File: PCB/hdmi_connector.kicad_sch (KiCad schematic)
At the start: 4 parts, among them J4 HDMI_A_1.4, U11 PTN3360DBS_518

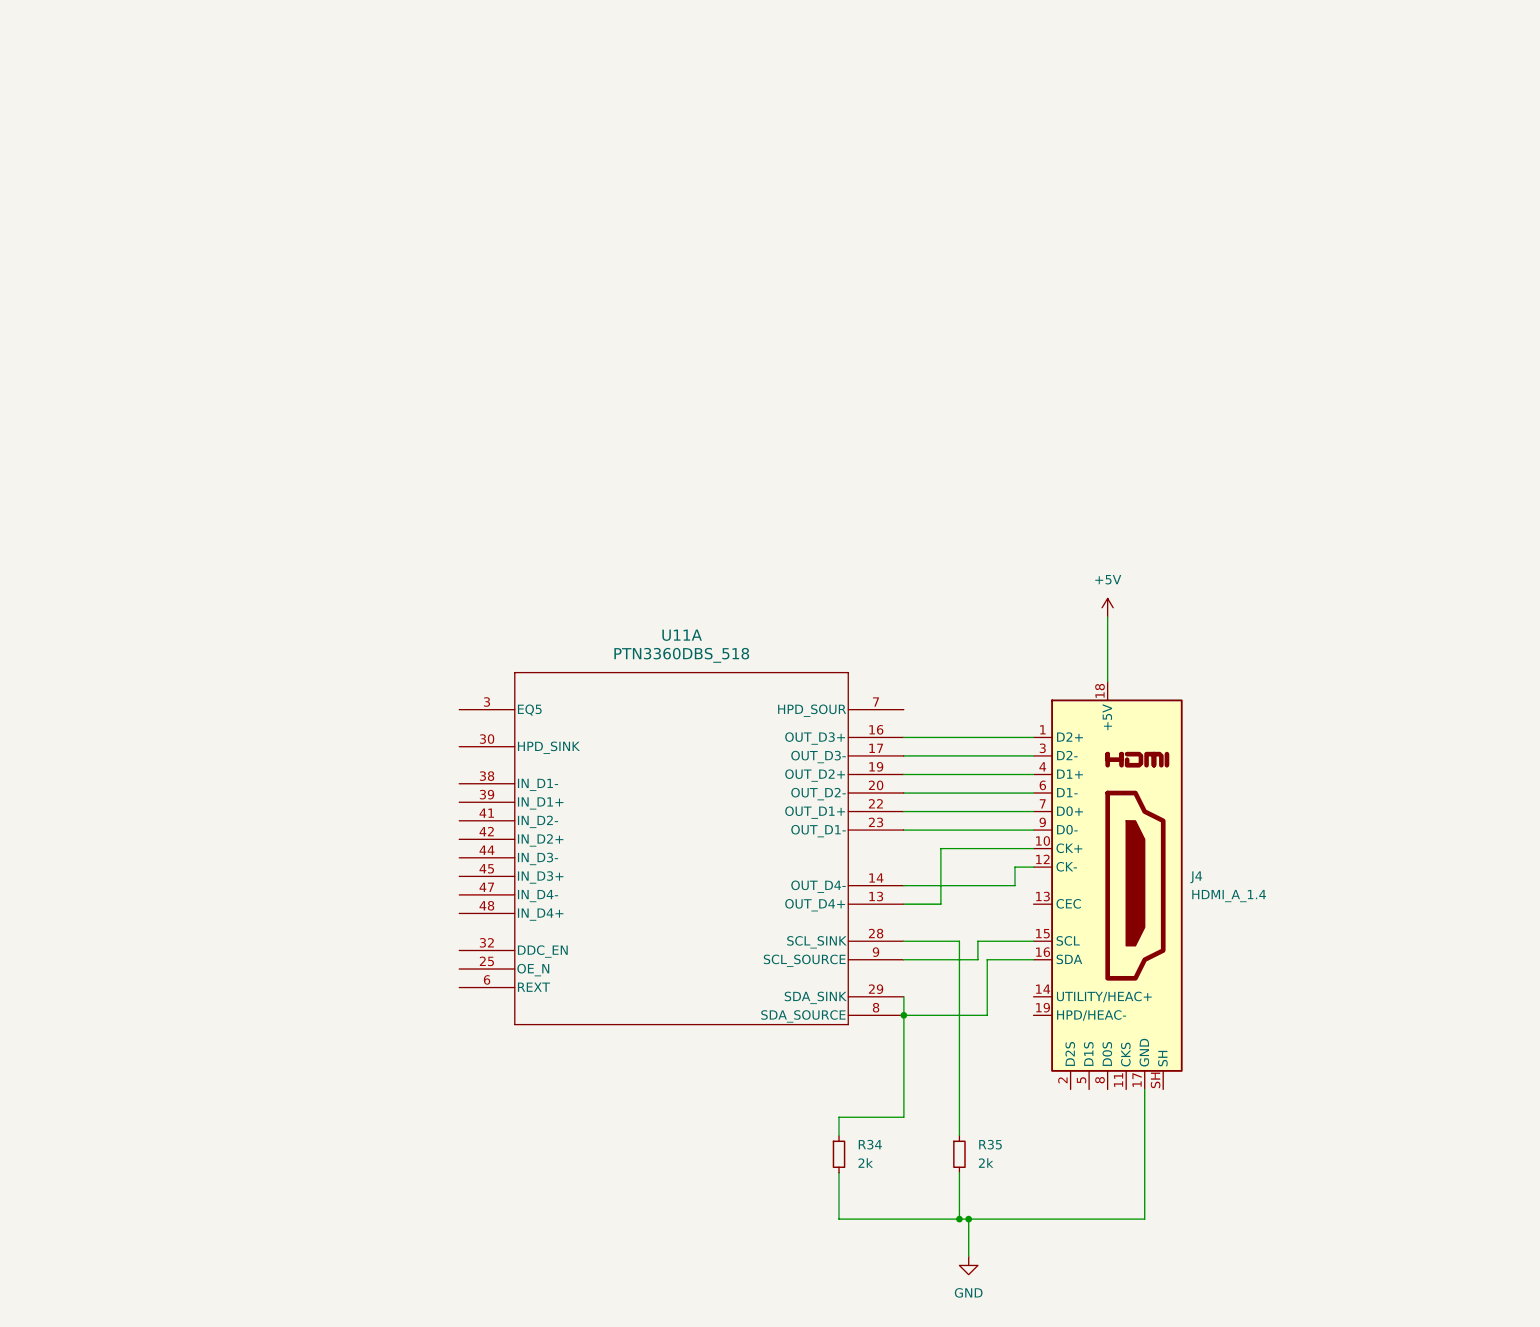
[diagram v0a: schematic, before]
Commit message: hdmi fix
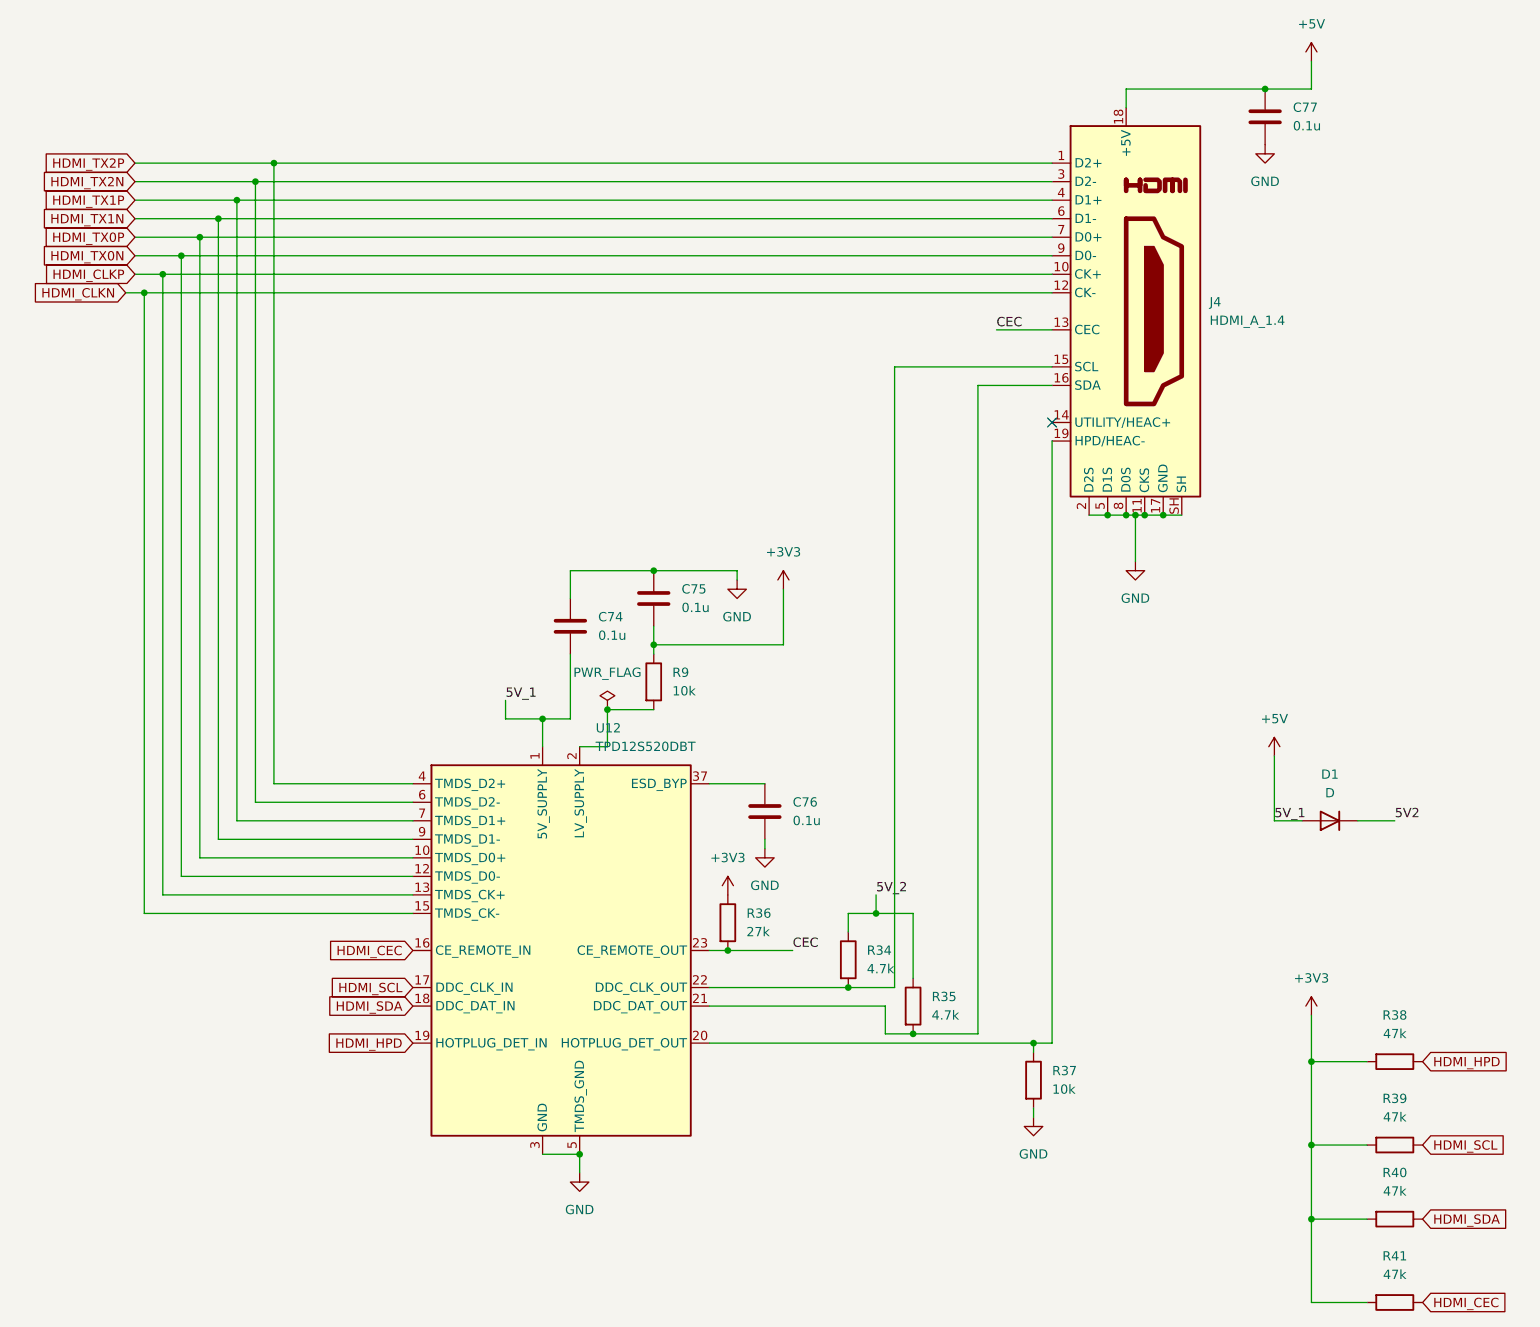
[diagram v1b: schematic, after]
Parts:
- removed R34, R35: 2k, symbol Device:R_Small
- removed U11: PTN3360DBS_518, HVQFN48_SOT619-1_NXP, symbol NXP_hdmi:PTN3360DBS_518
- added C74, C75, C76, C77: 0.1u, symbol Device:C
- added D1: D, symbol Device:D
- added R34, R35: 4.7k, symbol Device:R
- added R36: 27k, symbol Device:R
- added R37, R9: 10k, symbol Device:R
- added R38, R39, R40, R41: 47k, symbol Device:R
- added U12: TPD12S520DBT, Package_SO:TSSOP-38_4.4x9.7mm_P0.5mm, symbol Interface_HDMI:TPD12S520DBT
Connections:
- net +5V: now also C74.2, C77.1, D1.2 (A), U12.1 (5V_SUPPLY)
- net GND: now also J4.11 (CKS), J4.2 (D2S), J4.5 (D1S), J4.8 (D0S), J4.SH, C74.1, C75.1, C76.2, C77.2, R37.2, U12.11 (TMDS_GND), U12.14 (TMDS_GND), U12.25 (TMDS_GND), U12.28 (TMDS_GND), U12.3 (GND), U12.31 (TMDS_GND), U12.34 (TMDS_GND), U12.36 (GND), U12.5 (TMDS_GND), U12.8 (TMDS_GND)
- net HDMI_TX2P: now reaches J4.1 (D2+)
- net HDMI_TX2P: now also U12.35 (TMDS_D2+), U12.4 (TMDS_D2+)
- net HDMI_CLKP: now reaches J4.10 (CK+)
- net HDMI_CLKP: now also U12.13 (TMDS_CK+), U12.26 (TMDS_CK+)
- net HDMI_CLKN: now reaches J4.12 (CK-)
- net HDMI_CLKN: now also U12.15 (TMDS_CK-), U12.24 (TMDS_CK-)
- net CEC: now reaches J4.13 (CEC)
- net CEC: now also R36.2, U12.23 (CE_REMOTE_OUT)
- net at J4.15 (SCL): now also R34.2, U12.22 (DDC_CLK_OUT)
- net at J4.16 (SDA): now also R35.2, U12.21 (DDC_DAT_OUT)
- net at J4.19 (HPD/HEAC-): now also R37.1, U12.20 (HOTPLUG_DET_OUT)
- net HDMI_TX2N: now reaches J4.3 (D2-)
- net HDMI_TX2N: now also U12.33 (TMDS_D2-), U12.6 (TMDS_D2-)
- net HDMI_TX1P: now reaches J4.4 (D1+)
- net HDMI_TX1P: now also U12.32 (TMDS_D1+), U12.7 (TMDS_D1+)
- net HDMI_TX1N: now reaches J4.6 (D1-)
- net HDMI_TX1N: now also U12.30 (TMDS_D1-), U12.9 (TMDS_D1-)
- net HDMI_TX0P: now reaches J4.7 (D0+)
- net HDMI_TX0P: now also U12.10 (TMDS_D0+), U12.29 (TMDS_D0+)
- net HDMI_TX0N: now reaches J4.9 (D0-)
- net HDMI_TX0N: now also U12.12 (TMDS_D0-), U12.27 (TMDS_D0-)
- new net: C76.1, U12.37 (ESD_BYP)
- new net: R9.2, U12.2 (LV_SUPPLY)
- new net +3V3: C75.2, R36.1, R38.2, R39.2, R40.2, R41.2, R9.1
- new net 5V2: D1.1 (K)
- new net 5V_2: R34.1, R35.1
- new net HDMI_CEC: R41.1, U12.16 (CE_REMOTE_IN)
- new net HDMI_HPD: R38.1, U12.19 (HOTPLUG_DET_IN)
- new net HDMI_SCL: R39.1, U12.17 (DDC_CLK_IN)
- new net HDMI_SDA: R40.1, U12.18 (DDC_DAT_IN)
- no-connect marks 0 -> 1
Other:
- moved on the sheet: J4
